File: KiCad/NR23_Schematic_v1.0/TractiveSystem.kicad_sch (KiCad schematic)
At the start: 4 parts

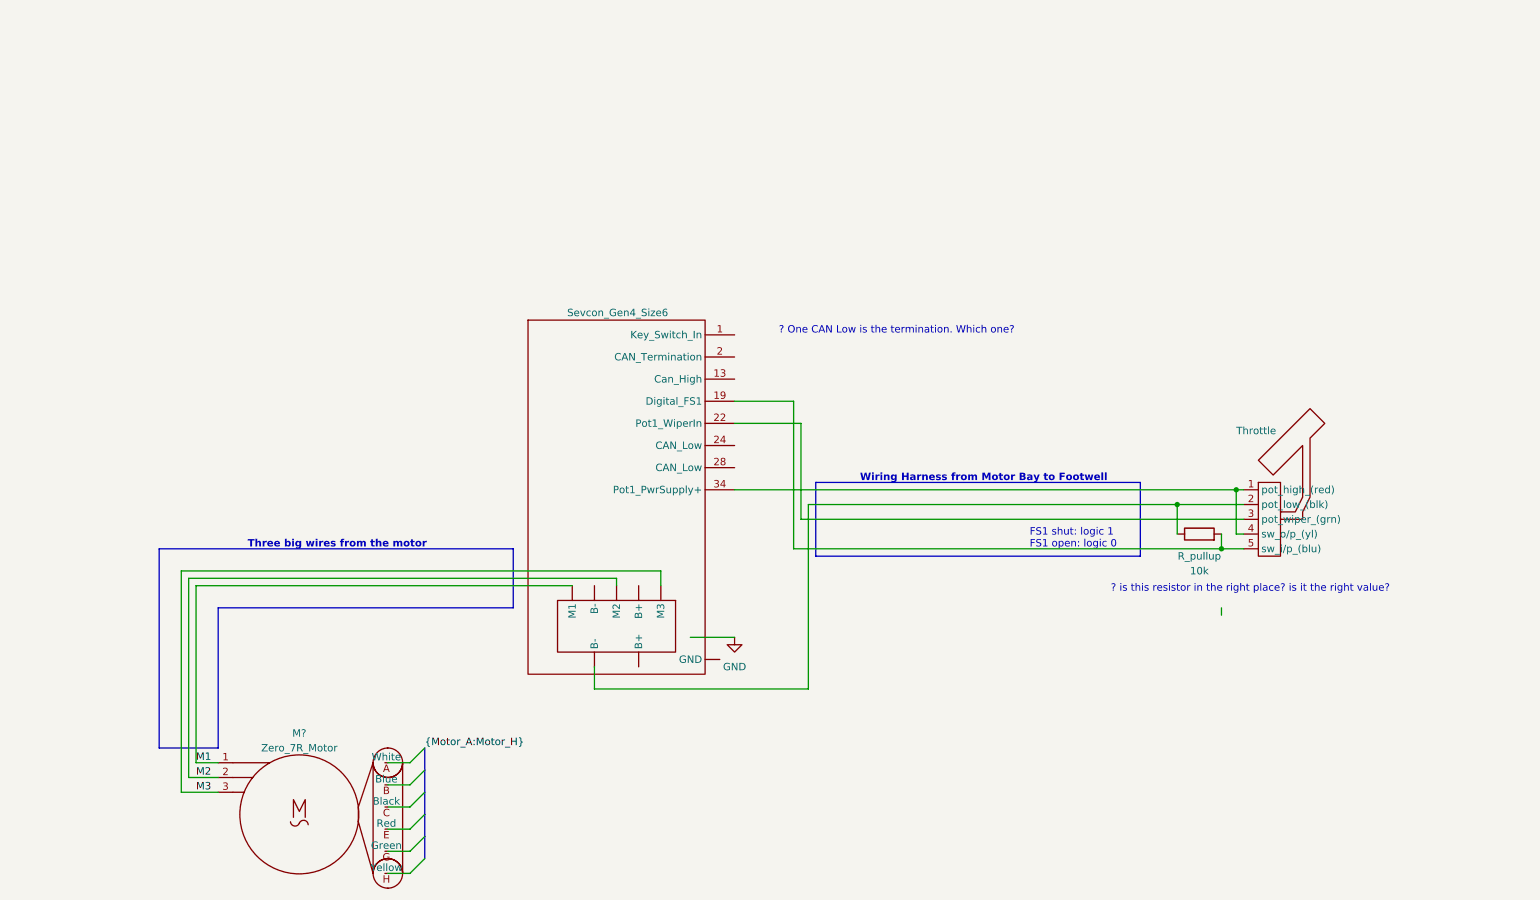
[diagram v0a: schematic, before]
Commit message: end of class 07FEB23
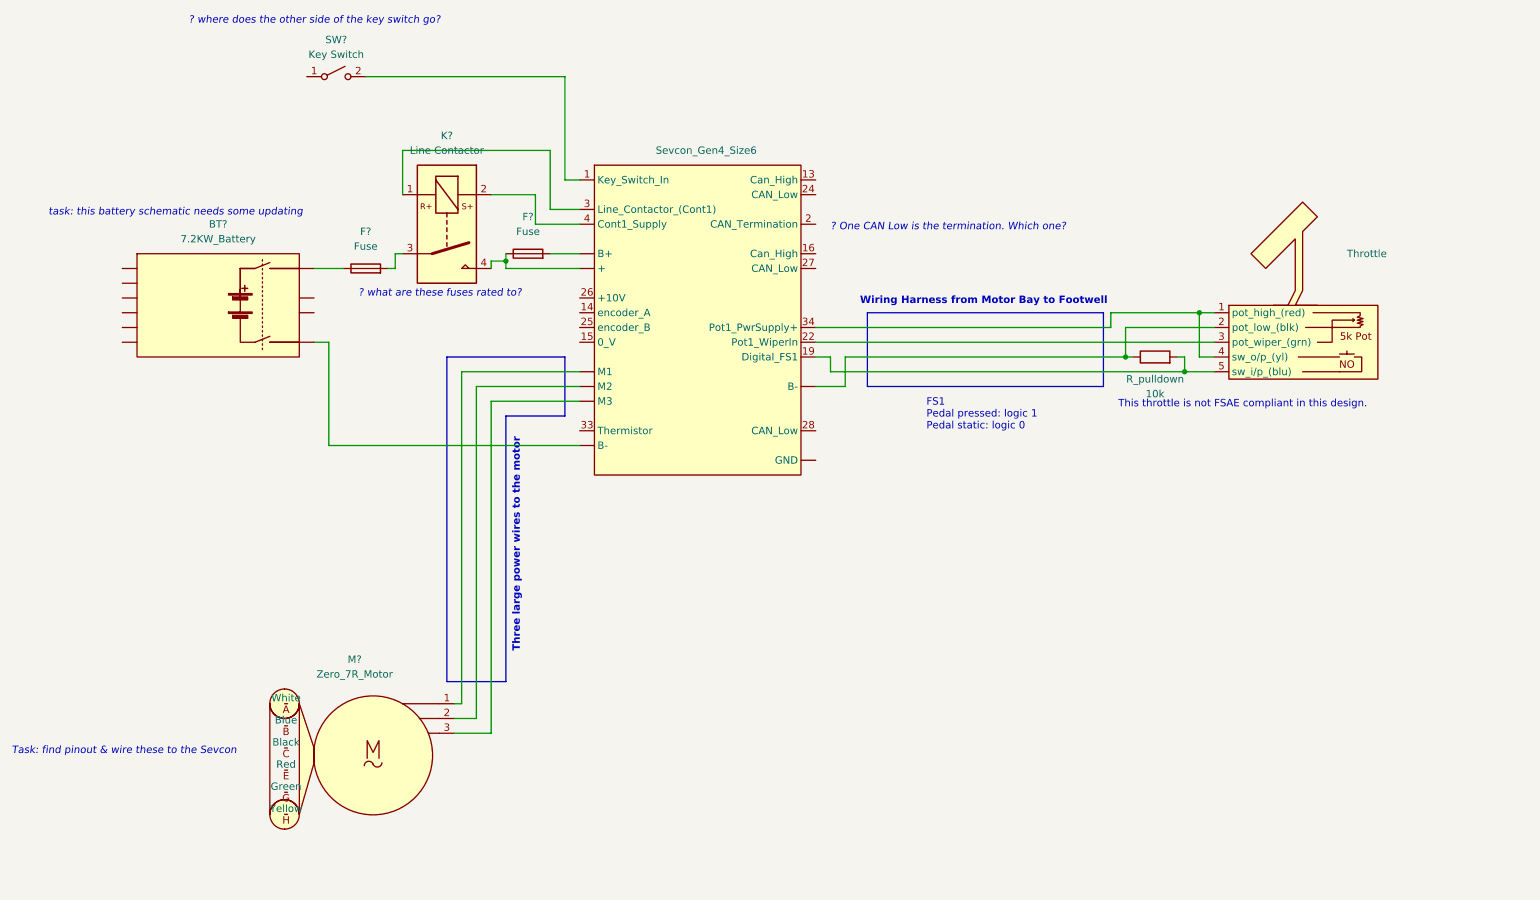
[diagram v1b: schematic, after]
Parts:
- added BT?: 7.2KW_Battery, symbol CamachosSymbols:7.2KW_Battery
- added F? (x2): Fuse, symbol Device:Fuse
- added K?: Line Contactor, Relay_THT:Relay_1P1T_NO_10x24x18.8mm_Panasonic_ADW11xxxxW_THT, symbol Relay:ADW11
- added SW?: Key Switch, symbol Switch:SW_SPST
- renumbered R_pullup to R_pulldown
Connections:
- net at U?. (M3): now also F?.2
- net at U?.1 (Key_Switch_In): now also SW?.2 (B)
- net M1: no longer names the net of M?.1, U?. (M3)
- net M2: no longer names the net of M?.2, U?. (M3)
- net M3: no longer names the net of M?.3, U?. (M3)
- new net: BT?.2 (-), U?. (M3)
- new net: F?.1, K?.4, U?. (M3)
- new net: K?.1, U?.3 (Line_Contactor_(Cont1))
- new net: K?.2, U?.4 (Cont1_Supply)
- new net: BT?.1 (+), F?.1
- new net: F?.2, K?.3
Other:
- note added: "? what are these fuses rated to?"
- note added: "? where does the other side of the key switch go?"
- note added: "FS1 Pedal pressed: logic 1 Pedal static: logic 0"
- note added: "Task: find pinout & wire these to the Sevcon"
- note added: "This throttle is not FSAE compliant in this design."
- note added: "Three large power wires to the motor"
- note added: "task: this battery schematic needs some updating"
- note removed: "? is this resistor in the right place? is it the right value?"
- note removed: "FS1 shut: logic 1 FS1 open: logic 0"
- note removed: "Three big wires from the motor"
- moved on the sheet: R_pulldown
